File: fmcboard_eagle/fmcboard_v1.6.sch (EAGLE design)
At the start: 294 parts, among them IC1 OPA699ID, IC10 LM358, IC11 7805DT, IC12 SN74AUC2G66DCTR, IC13 SN74AUC2G66DCTR, IC14 SN74AUC2G66DCTR, IC15 SN74AUC2G66DCTR, IC16 DAC7578SPWR, IC17 SN74AUC2G66DCTR, IC18 SN74AUC2G66DCTR, IC19 SN74AUC2G66DCTR, IC2 DAC7578SPWR, IC20 SN74AUC2G66DCTR, IC21 74AUP2GU04GW, IC22 74AUP2GU04GW, IC23 74AUP2GU04GW, IC24 74AUP2GU04GW, IC25 MC7905ACD2TR4G, IC26 AMS1117-1.8, IC27 LM358, IC28 SN74AUC2G66DCTR, IC29 LM337KVURG3, IC3 LTC6229IMS8E#TRPBF, IC30 SN74AUC2G66DCTR, IC31 SN74AUC2G66DCTR, IC32 SN74AUC2G66DCTR, IC33 LTC6229IMS8E#TRPBF, IC34 74AUP2GU04GW, IC35 74AUP2GU04GW, IC36 TPS5430DDAR, IC37 TPS5430DDAR, IC4 OPA695IDR, IC5 LTC6229IMS8E#TRPBF, IC6 OPA695IDR, IC7 OPA699ID, IC8 LM358, IC9 LM358, J1 8pin, J12 4p-2.54, J13 4p-2.54, J2 ASP-134604-01, J3 2p-2.54, J5 4p-2.54, J8 4p-2.54, J9 2p-2.54

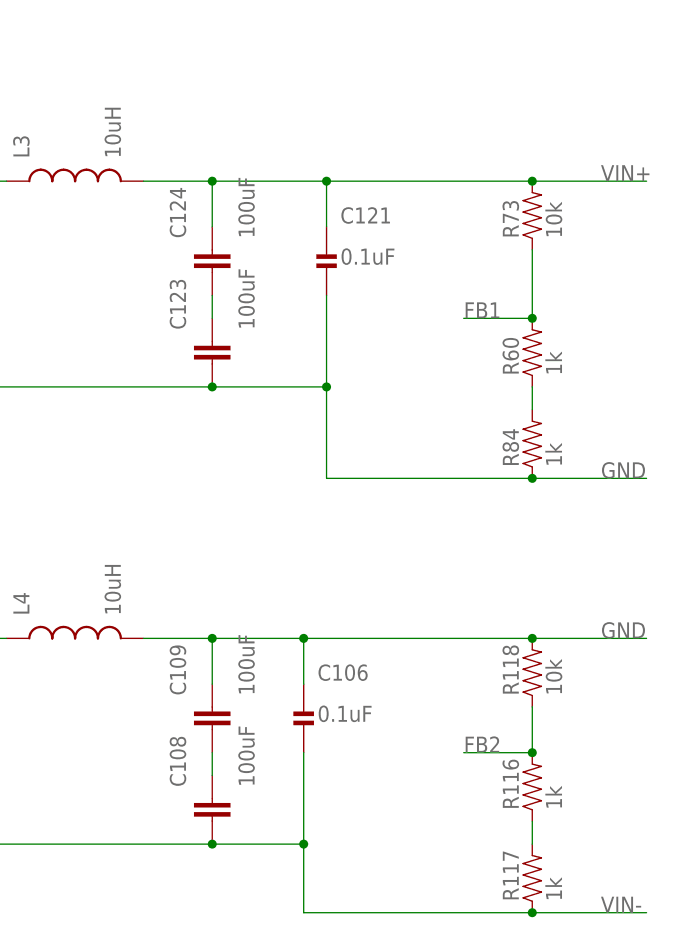
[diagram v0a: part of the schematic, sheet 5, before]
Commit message: tantalum 100uF
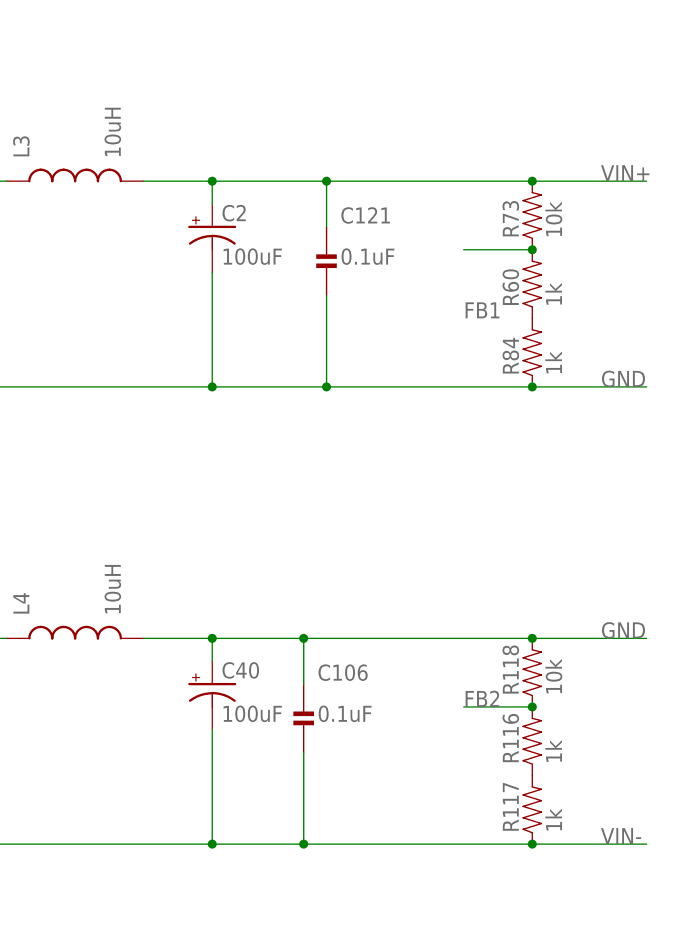
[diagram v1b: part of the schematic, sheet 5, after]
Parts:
- removed C108, C109, C123, C124: 100uF, rcl:C-EUC1206K
- added C2, C40: 100uF, SparkFun-Passives:CAP_POLSMD
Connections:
- removed net N$53: C123.1, C124.2
- removed net N$55: C108.1, C109.2
- net GND: now also C2.-, C40.+; no longer C109.1, C123.2
- net VIN+: now also C2.+; no longer C124.1
- net VIN-: now also C40.-; no longer C108.2
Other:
- moved on the sheet: R116, R117, R60, R84

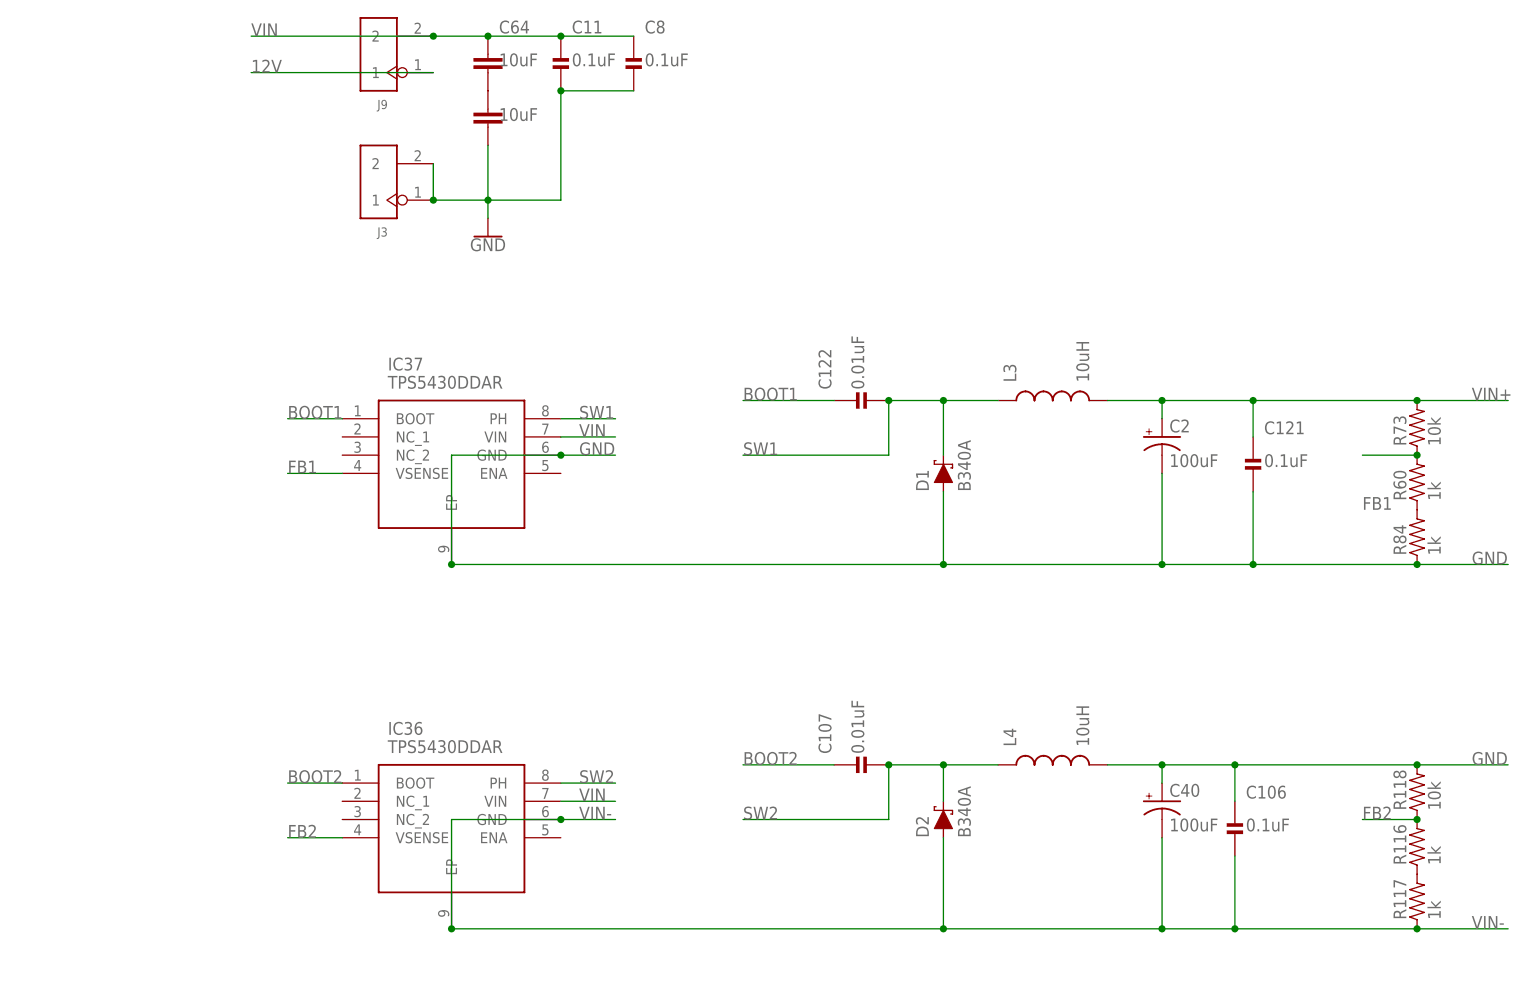
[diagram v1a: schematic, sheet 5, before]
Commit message: routed
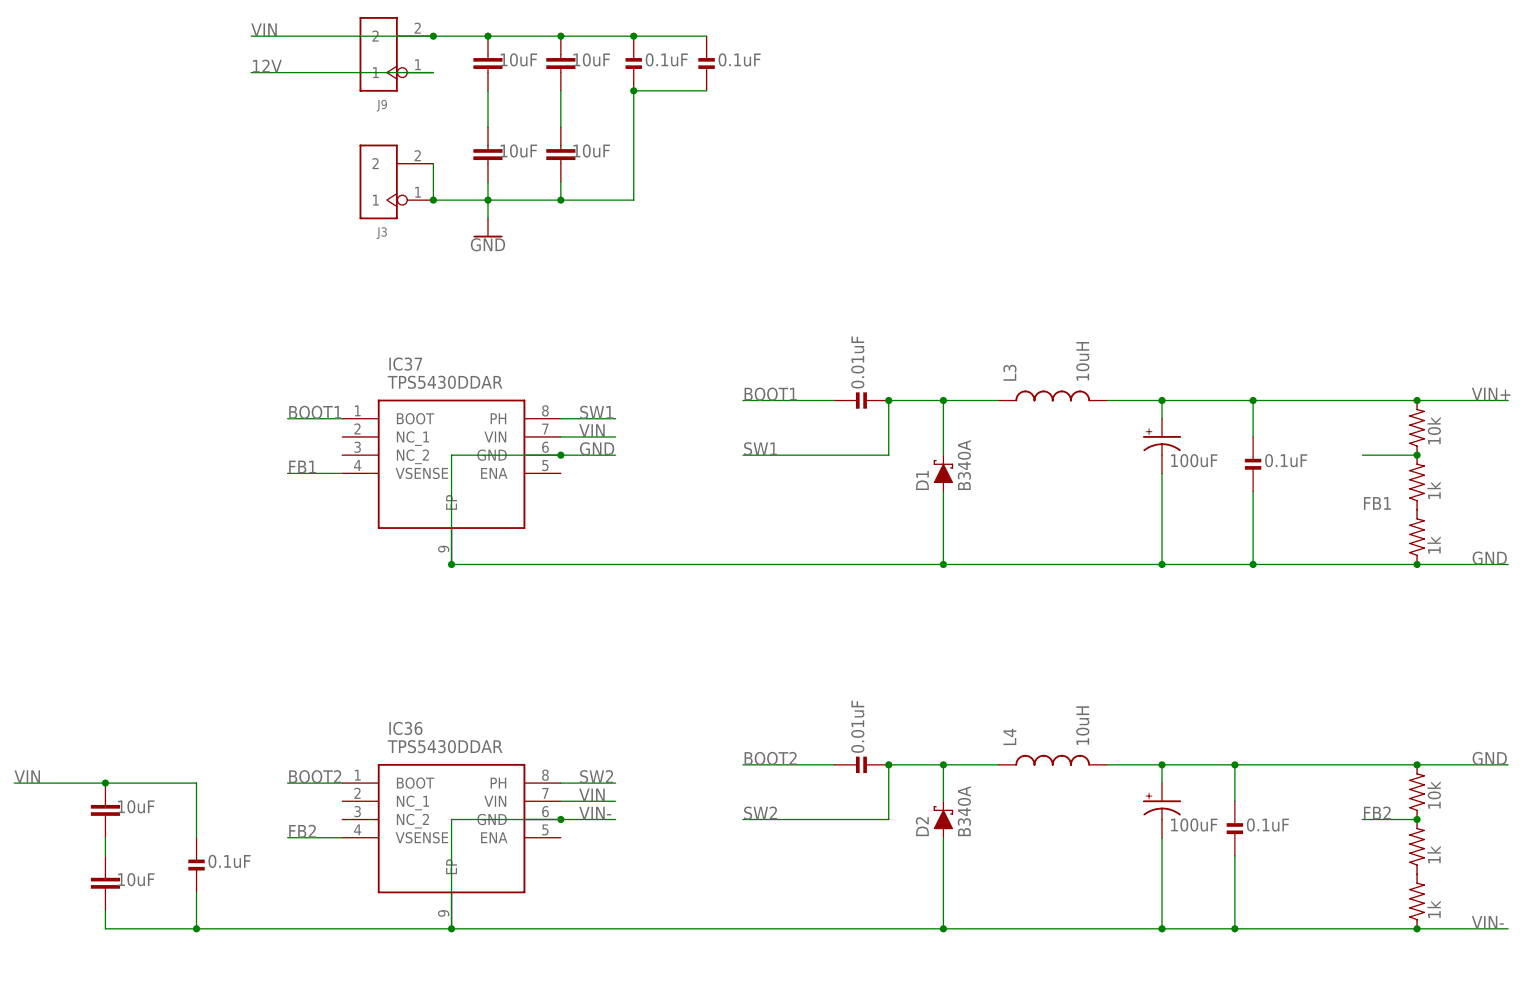
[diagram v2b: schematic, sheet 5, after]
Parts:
- added C108, C109, C112, C80: 10uF, rcl:C-EUC0805
- added C113: 0.1uF, passives:CAPACITOR0402_CAP
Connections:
- new net N$35: C108.1, C80.2
- new net N$53: C109.1, C112.2
- net GND: now also C108.2
- net VIN: now also C112.1, C113.1, C80.1
- net VIN-: now also C109.2, C113.2
